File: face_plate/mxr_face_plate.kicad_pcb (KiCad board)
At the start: 2 copper layers, 20 x 128.5 mm, 10 parts

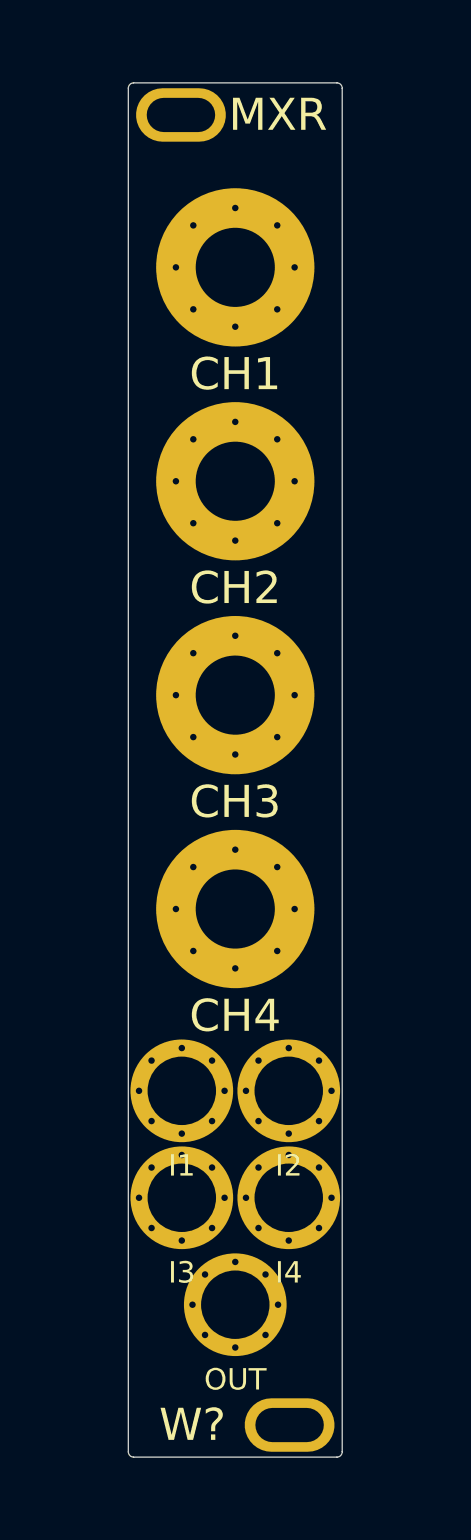
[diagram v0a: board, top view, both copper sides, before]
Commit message: faceplate
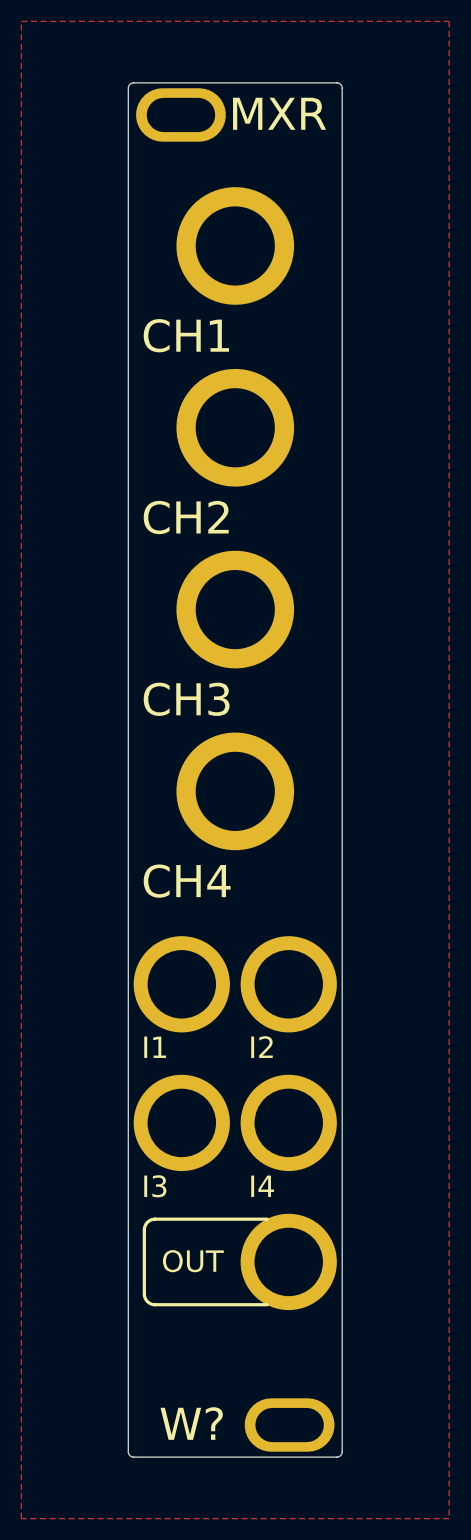
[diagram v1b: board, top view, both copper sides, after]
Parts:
- H101, H102, H103, H104: footprint WITNS:PotentiometerHole_7.4mm_M7_Pad_Via -> WITNS:PotentiometerHole_7.4mm_M7_Pad
- H105, H106, H107, H108, H109: footprint WITNS:Thonkiconn_6.4mm_M6_Pad_Via -> WITNS:Thonkiconn_6.4mm_M6_Pad
- moved H104 11.0 mm to (50.0, 102.0)
- moved H105 9.96 mm to (45.0, 120.0)
- moved H106 9.96 mm to (55.0, 120.0)
- moved H103 8.00 mm to (50.0, 85.0)
- moved H107 7.00 mm to (45.0, 133.0)
- moved H108 7.00 mm to (55.0, 133.0)
- moved H109 6.40 mm to (55.0, 146.0)
- moved H102 5.00 mm to (50.0, 68.0)
- moved H101 2.00 mm to (50.0, 51.0)
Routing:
- added copper zone on F.Cu, net GND
